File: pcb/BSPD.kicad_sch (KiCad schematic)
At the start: 42 parts, among them J1 Test header, J2 T4142012121-000, Q1 AO3400A, U1 LM339, U2 LM339, U3 74HC32, U4 LM339, U8 74HC1G04GV,125

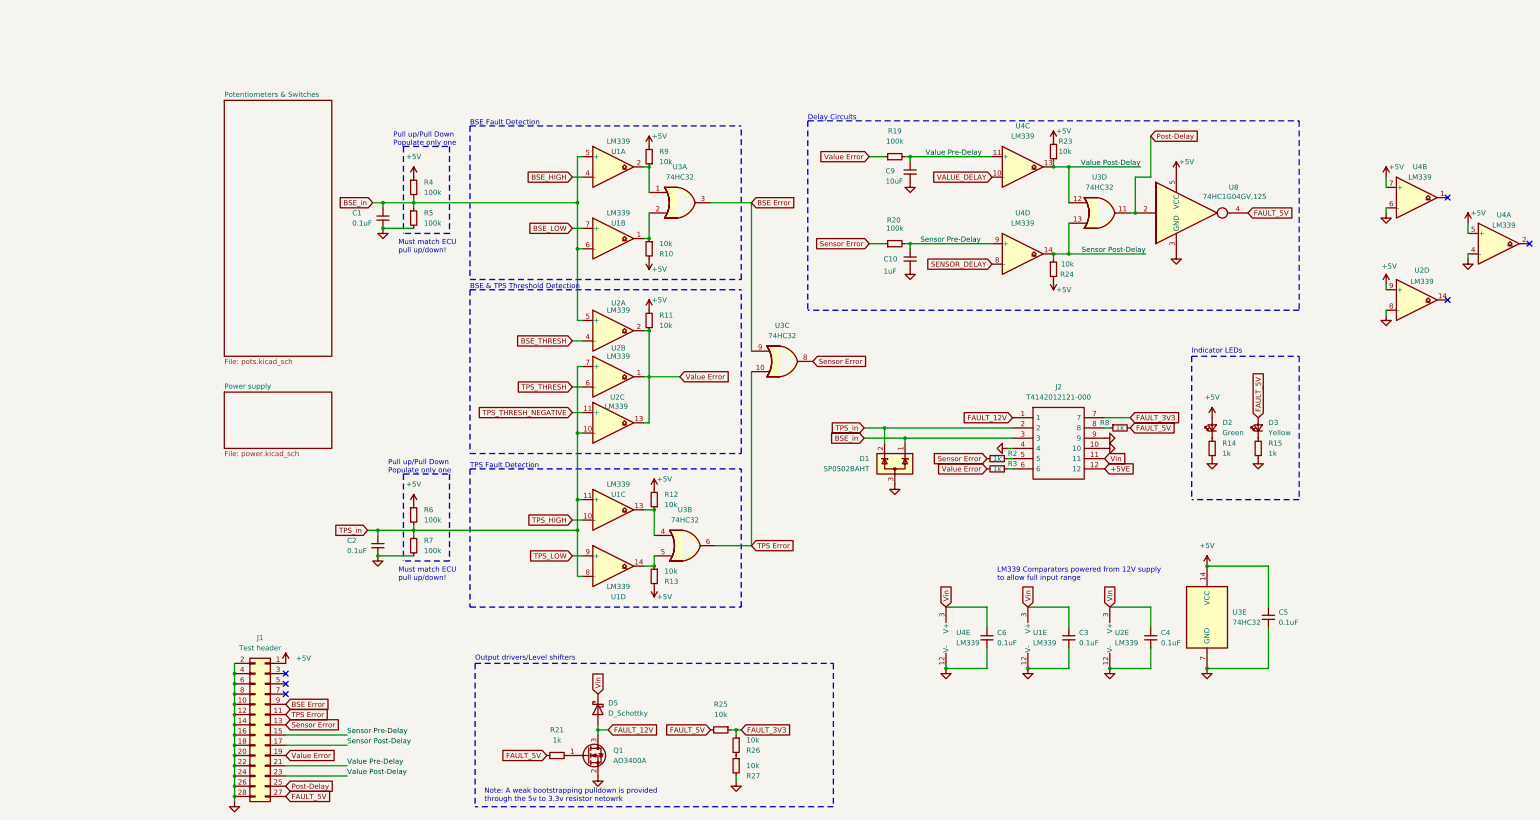
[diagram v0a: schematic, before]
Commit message: Remove lck files
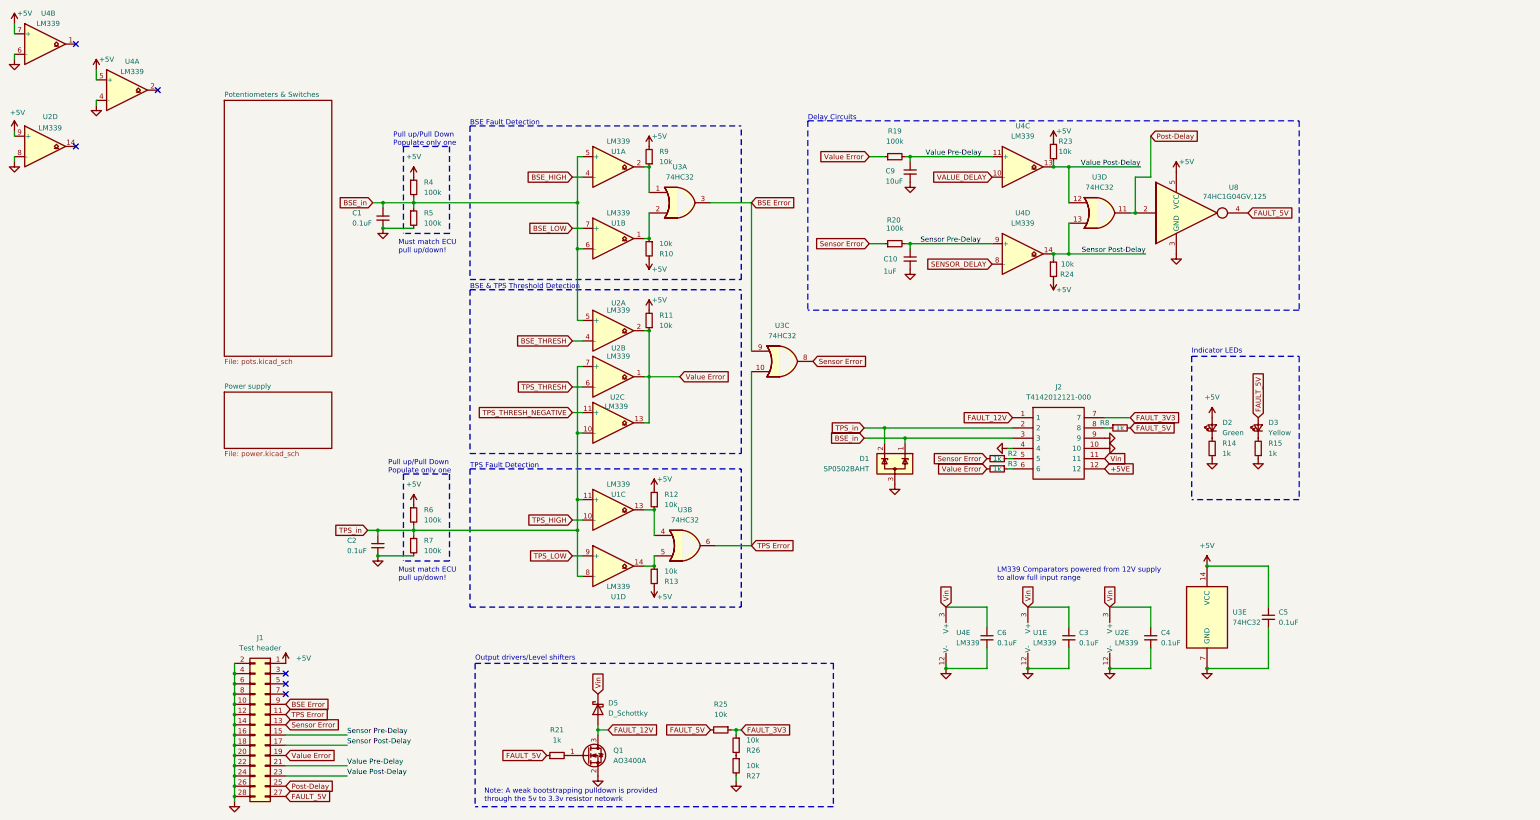
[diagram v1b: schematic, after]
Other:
- moved on the sheet: U2D, U4A, U4B
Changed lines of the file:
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@@
 	)
 	(no_connect
-		(at 339.09 53.34)
+		(at -1.27 15.24)
 	)
 	(no_connect
@@
 	)
 	(no_connect
-		(at 318.77 41.91)
+		(at -21.59 3.81)
 	)
 	(no_connect
-		(at 318.77 67.31)
+		(at -21.59 29.21)
 	)
 	(polyline
@@
 	(wire
 		(pts
-			(xy 303.53 63.5) (xy 303.53 64.77)
+			(xy -36.83 25.4) (xy -36.83 26.67)
 		)
 		(stroke
@@
 	(wire
 		(pts
-			(xy 323.85 48.26) (xy 323.85 50.8)
+			(xy -16.51 10.16) (xy -16.51 12.7)
 		)
 		(stroke
@@
 	(wire
 		(pts
-			(xy 303.53 71.12) (xy 303.53 69.85)
+			(xy -36.83 33.02) (xy -36.83 31.75)
 		)
 		(stroke
@@
 	(wire
 		(pts
-			(xy 323.85 57.15) (xy 323.85 55.88)
+			(xy -16.51 19.05) (xy -16.51 17.78)
 		)
 		(stroke
@@
 	(wire
 		(pts
-			(xy 303.53 44.45) (xy 303.53 45.72)
+			(xy -36.83 6.35) (xy -36.83 7.62)
 		)
 		(stroke
@@
 	(wire
 		(pts
-			(xy 303.53 36.83) (xy 303.53 39.37)
+			(xy -36.83 -1.27) (xy -36.83 1.27)
 		)
 		(stroke
@@
 	(symbol
 		(lib_id "Comparator:LM339")
-		(at 331.47 53.34 0)
+		(at -8.89 15.24 0)
 		(unit 1)
 		(exclude_from_sim no)
@@
 		(dnp no)
 		(property "Reference" "U4"
-			(at 332.74 46.228 0)
+			(at -7.62 8.128 0)
 			(effects
 				(font
@@
 		)
 		(property "Value" "LM339"
-			(at 332.74 48.768 0)
+			(at -7.62 10.668 0)
 			(effects
 				(font
@@
 		)
 		(property "Footprint" "Package_SO:SOIC-14_3.9x8.7mm_P1.27mm"
-			(at 330.2 50.8 0)
+			(at -10.16 12.7 0)
 			(effects
 				(font
@@
 		)
 		(property "Datasheet" "https://www.st.com/resource/en/datasheet/lm139.pdf"
-			(at 332.74 48.26 0)
+			(at -7.62 10.16 0)
 			(effects
 				(font
@@
 		)
 		(property "Description" "Quad Differential Comparators, SOIC-14/TSSOP-14"
-			(at 331.47 53.34 0)
+			(at -8.89 15.24 0)
 			(effects
 				(font
@@
 	(symbol
 		(lib_id "power:+5V")
-		(at 303.53 36.83 0)
+		(at -36.83 -1.27 0)
 		(unit 1)
 		(exclude_from_sim no)
@@
 		(dnp no)
 		(property "Reference" "#PWR022"
-			(at 303.53 40.64 0)
+			(at -36.83 2.54 0)
 			(effects
 				(font
@@
 		)
 		(property "Value" "+5V"
-			(at 306.07 34.29 0)
+			(at -34.29 -3.81 0)
 			(effects
 				(font
@@
 		)
 		(property "Footprint" ""
-			(at 303.53 36.83 0)
+			(at -36.83 -1.27 0)
 			(effects
 				(font
@@
 		)
 		(property "Datasheet" ""
-			(at 303.53 36.83 0)
+			(at -36.83 -1.27 0)
 			(effects
 				(font
@@
 		)
 		(property "Description" "Power symbol creates a global label with name \"+5V\""
-			(at 303.53 36.83 0)
+			(at -36.83 -1.27 0)
 			(effects
 				(font
@@
 	(symbol
 		(lib_id "Comparator:LM339")
-		(at 311.15 67.31 0)
+		(at -29.21 29.21 0)
 		(unit 4)
 		(exclude_from_sim no)
@@
 		(dnp no)
 		(property "Reference" "U2"
-			(at 312.42 59.944 0)
+			(at -27.94 21.844 0)
 			(effects
 				(font
@@
 		)
 		(property "Value" "LM339"
-			(at 312.42 62.738 0)
+			(at -27.94 24.638 0)
 			(effects
 				(font
@@
 		)
 		(property "Footprint" "Package_SO:SOIC-14_3.9x8.7mm_P1.27mm"
-			(at 309.88 64.77 0)
+			(at -30.48 26.67 0)
 			(effects
 				(font
@@
 		)
 		(property "Datasheet" "https://www.st.com/resource/en/datasheet/lm139.pdf"
-			(at 312.42 62.23 0)
+			(at -27.94 24.13 0)
 			(effects
 				(font
@@
 		)
 		(property "Description" "Quad Differential Comparators, SOIC-14/TSSOP-14"
-			(at 311.15 67.31 0)
+			(at -29.21 29.21 0)
 			(effects
 				(font
@@
 		)
 		(property "LCSC" "C63821"
-			(at 311.15 67.31 0)
+			(at -29.21 29.21 0)
 			(effects
 				(font
@@
 		)
 		(property "Sim.Device" "SPICE"
-			(at 180.34 36.83 0)
+			(at -160.02 -1.27 0)
 			(effects
 				(font
@@
 		)
 		(property "Sim.Params" "type=\"X\" model=\"LM339\" lib=\"SPICE models/lmx39_spice.lib\""
-			(at 77.47 40.64 0)
+			(at -262.89 2.54 0)
 			(effects
 				(font
@@
 		)
 		(property "Sim.Pins" "1=1 2=2 3=3 4=4 5=5 6=6 7=7 8=8 9=9 10=10 11=11 12=12 13=13 14=14"
-			(at 77.47 40.64 0)
+			(at -262.89 2.54 0)
 			(effects
 				(font
@@
 	(symbol
 		(lib_id "power:GND")
-		(at 303.53 71.12 0)
+		(at -36.83 33.02 0)
 		(unit 1)
 		(exclude_from_sim no)
@@
 		(fields_autoplaced yes)
 		(property "Reference" "#PWR034"
-			(at 303.53 77.47 0)
+			(at -36.83 39.37 0)
 			(effects
 				(font
@@
 		)
 		(property "Value" "GND"
-			(at 303.53 76.2 0)
+			(at -36.83 38.1 0)
 			(effects
 				(font
@@
 		)
 		(property "Footprint" ""
-			(at 303.53 71.12 0)
+			(at -36.83 33.02 0)
 			(effects
 				(font
@@
 		)
 		(property "Datasheet" ""
-			(at 303.53 71.12 0)
+			(at -36.83 33.02 0)
 			(effects
 				(font
@@
 		)
 		(property "Description" "Power symbol creates a global label with name \"GND\" , ground"
-			(at 303.53 71.12 0)
+			(at -36.83 33.02 0)
 			(effects
 				(font
@@
 	(symbol
 		(lib_id "power:+5V")
-		(at 303.53 63.5 0)
+		(at -36.83 25.4 0)
 		(unit 1)
 		(exclude_from_sim no)
@@
 		(dnp no)
 		(property "Reference" "#PWR032"
-			(at 303.53 67.31 0)
+			(at -36.83 29.21 0)
 			(effects
 				(font
@@
 		)
 		(property "Value" "+5V"
-			(at 304.292 58.928 0)
+			(at -36.068 20.828 0)
 			(effects
 				(font
@@
 		)
 		(property "Footprint" ""
-			(at 303.53 63.5 0)
+			(at -36.83 25.4 0)
 			(effects
 				(font
@@
 		)
 		(property "Datasheet" ""
-			(at 303.53 63.5 0)
+			(at -36.83 25.4 0)
 			(effects
 				(font
@@
 		)
 		(property "Description" "Power symbol creates a global label with name \"+5V\""
-			(at 303.53 63.5 0)
+			(at -36.83 25.4 0)
 			(effects
 				(font
@@
 	(symbol
 		(lib_id "power:GND")
-		(at 323.85 57.15 0)
+		(at -16.51 19.05 0)
 		(unit 1)
 		(exclude_from_sim no)
@@
 		(fields_autoplaced yes)
 		(property "Reference" "#PWR038"
-			(at 323.85 63.5 0)
+			(at -16.51 25.4 0)
 			(effects
 				(font
@@
 		)
 		(property "Value" "GND"
-			(at 323.85 62.23 0)
+			(at -16.51 24.13 0)
 			(effects
 				(font
@@
 		)
 		(property "Footprint" ""
-			(at 323.85 57.15 0)
+			(at -16.51 19.05 0)
 			(effects
 				(font
@@
 		)
 		(property "Datasheet" ""
-			(at 323.85 57.15 0)
+			(at -16.51 19.05 0)
 			(effects
 				(font
@@
 		)
 		(property "Description" "Power symbol creates a global label with name \"GND\" , ground"
-			(at 323.85 57.15 0)
+			(at -16.51 19.05 0)
 			(effects
 				(font
@@
 	(symbol
 		(lib_id "power:GND")
-		(at 303.53 45.72 0)
+		(at -36.83 7.62 0)
 		(unit 1)
 		(exclude_from_sim no)
@@
 		(fields_autoplaced yes)
 		(property "Reference" "#PWR039"
-			(at 303.53 52.07 0)
+			(at -36.83 13.97 0)
 			(effects
 				(font
@@
 		)
 		(property "Value" "GND"
-			(at 303.53 50.8 0)
+			(at -36.83 12.7 0)
 			(effects
 				(font
@@
 		)
 		(property "Footprint" ""
-			(at 303.53 45.72 0)
+			(at -36.83 7.62 0)
 			(effects
 				(font
@@
 		)
 		(property "Datasheet" ""
-			(at 303.53 45.72 0)
+			(at -36.83 7.62 0)
 			(effects
 				(font
@@
 		)
 		(property "Description" "Power symbol creates a global label with name \"GND\" , ground"
-			(at 303.53 45.72 0)
+			(at -36.83 7.62 0)
 			(effects
 				(font
@@
 	(symbol
 		(lib_id "power:+5V")
-		(at 323.85 48.26 0)
+		(at -16.51 10.16 0)
 		(unit 1)
 		(exclude_from_sim no)
@@
 		(dnp no)
 		(property "Reference" "#PWR029"
-			(at 323.85 52.07 0)
+			(at -16.51 13.97 0)
 			(effects
 				(font
@@
 		)
 		(property "Value" "+5V"
-			(at 326.39 45.72 0)
+			(at -13.97 7.62 0)
 			(effects
 				(font
@@
 		)
 		(property "Footprint" ""
-			(at 323.85 48.26 0)
+			(at -16.51 10.16 0)
 			(effects
 				(font
@@
 		)
 		(property "Datasheet" ""
-			(at 323.85 48.26 0)
+			(at -16.51 10.16 0)
 			(effects
 				(font
@@
 		)
 		(property "Description" "Power symbol creates a global label with name \"+5V\""
-			(at 323.85 48.26 0)
+			(at -16.51 10.16 0)
 			(effects
 				(font
@@
 	(symbol
 		(lib_id "Comparator:LM339")
-		(at 311.15 41.91 0)
+		(at -29.21 3.81 0)
 		(unit 2)
 		(exclude_from_sim no)
@@
 		(dnp no)
 		(property "Reference" "U4"
-			(at 311.912 34.29 0)
+			(at -28.448 -3.81 0)
 			(effects
 				(font
@@
 		)
 		(property "Value" "LM339"
-			(at 311.912 36.83 0)
+			(at -28.448 -1.27 0)
 			(effects
 				(font
@@
 		)
 		(property "Footprint" "Package_SO:SOIC-14_3.9x8.7mm_P1.27mm"
-			(at 309.88 39.37 0)
+			(at -30.48 1.27 0)
 			(effects
 				(font
@@
 		)
 		(property "Datasheet" "https://www.st.com/resource/en/datasheet/lm139.pdf"
-			(at 312.42 36.83 0)
+			(at -27.94 -1.27 0)
 			(effects
 				(font
@@
 		)
 		(property "Description" "Quad Differential Comparators, SOIC-14/TSSOP-14"
-			(at 311.15 41.91 0)
+			(at -29.21 3.81 0)
 			(effects
 				(font
